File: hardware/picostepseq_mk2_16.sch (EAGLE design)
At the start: 55 parts, among them J1 SJ-3523-SMT, J2 SJ-3523-SMT, SW1 LED_SWITCHSTEP, SW10 LED_SWITCHSTEP, SW11 LED_SWITCHSTEP, SW12 LED_SWITCHSTEP, SW13 LED_SWITCHSTEP, SW14 LED_SWITCHSTEP, SW15 LED_SWITCHSTEP, SW16 LED_SWITCHSTEP, SW17 LED_SWITCHSTEP, SW18 LED_SWITCHSTEP, SW2 LED_SWITCHSTEP, SW3 LED_SWITCHSTEP, SW4 LED_SWITCHSTEP, SW5 LED_SWITCHSTEP, SW6 LED_SWITCHSTEP, SW7 LED_SWITCHSTEP, SW8 LED_SWITCHSTEP, SW9 LED_SWITCHSTEP, U2 6N137, U3 WS2811-SOP8, U4 WS2811-SOP8, U5 WS2811-SOP8, U6 WS2811-SOP8, U7 WS2811-SOP8, U8 WS2811-SOP8

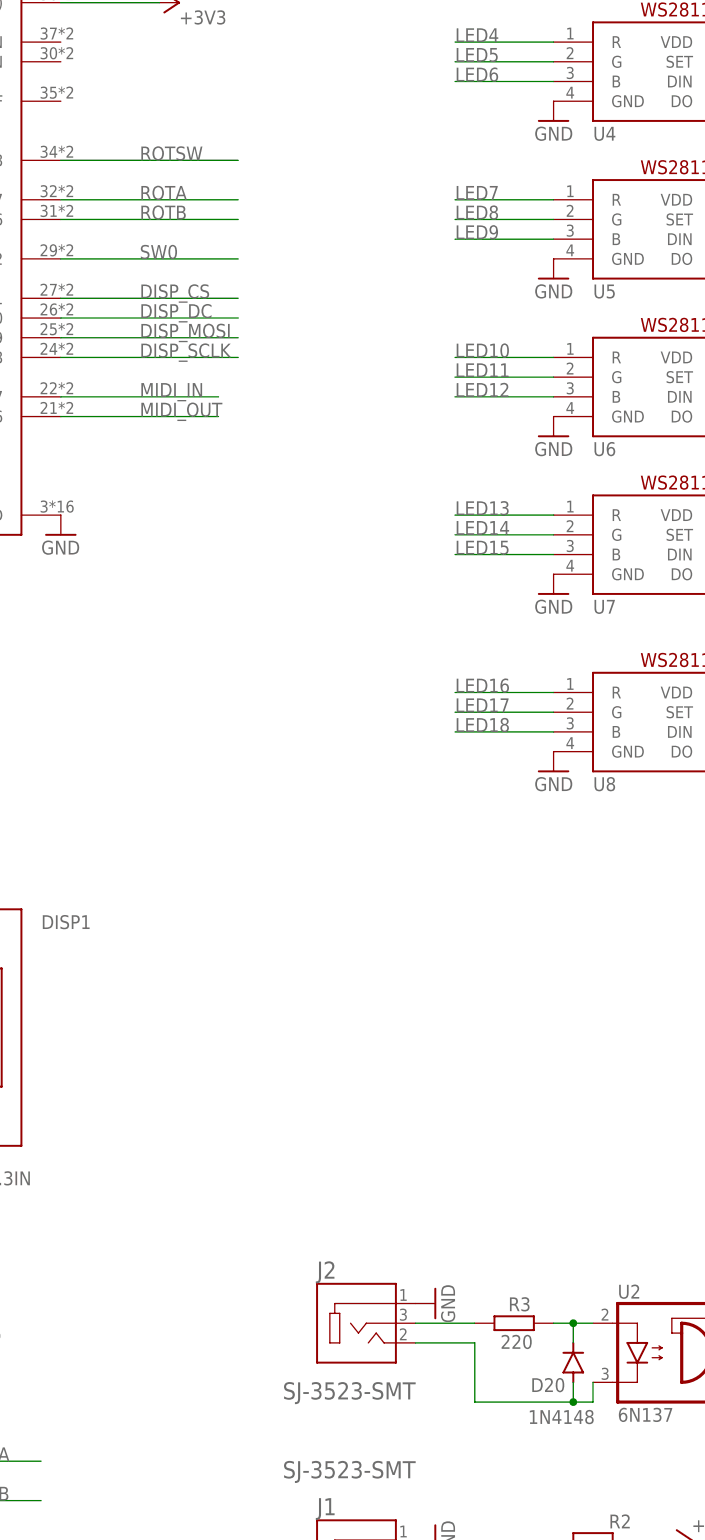
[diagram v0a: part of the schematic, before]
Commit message: "finish" picostepseq_mk2_16
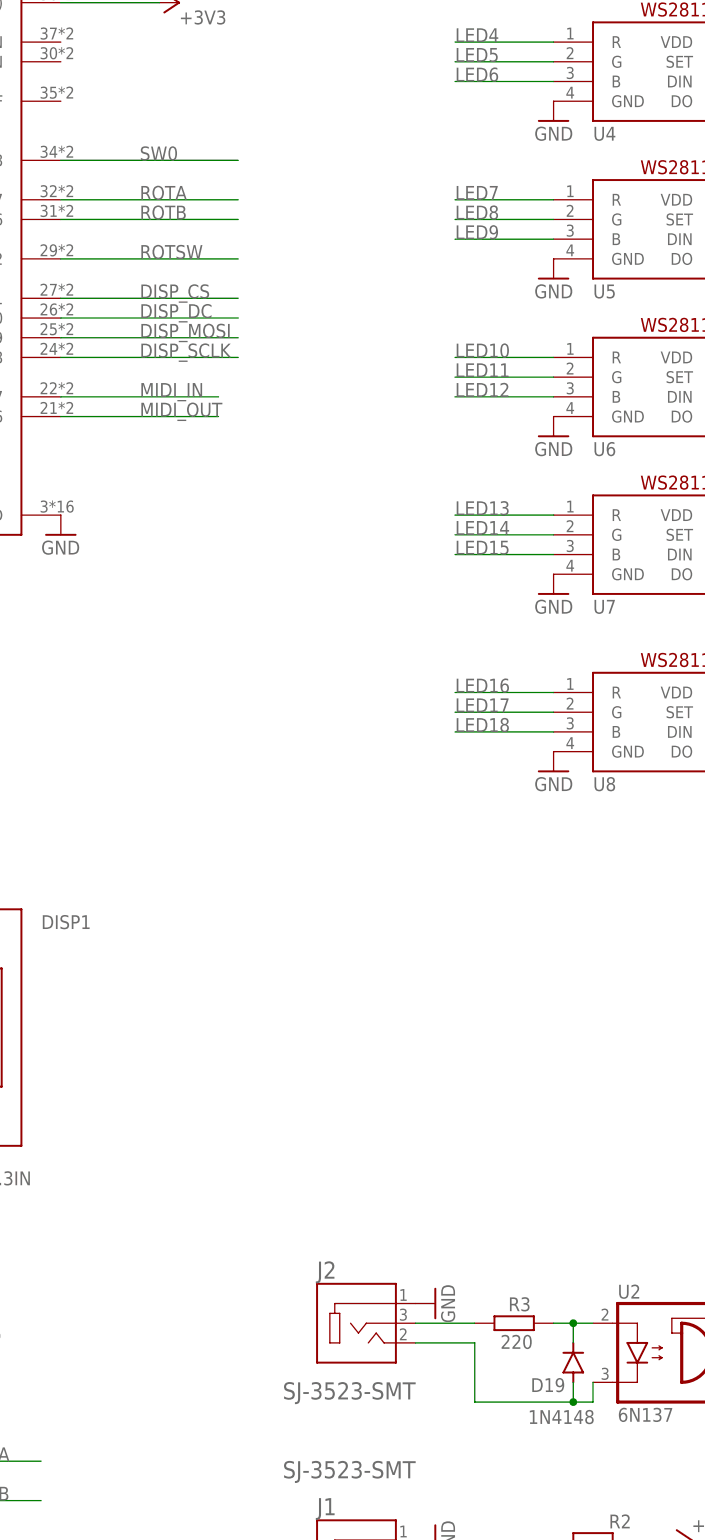
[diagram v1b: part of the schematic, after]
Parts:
- renumbered D20 to D19
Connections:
- net ROTSW: now also U1.GP22; no longer U1.GP28
- net SW0: now also U1.GP28; no longer U1.GP22
